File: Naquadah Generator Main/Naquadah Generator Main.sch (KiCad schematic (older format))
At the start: 15 parts, among them SW1 RESET, U1 ATmega32U4-AU, Y1 16MHz

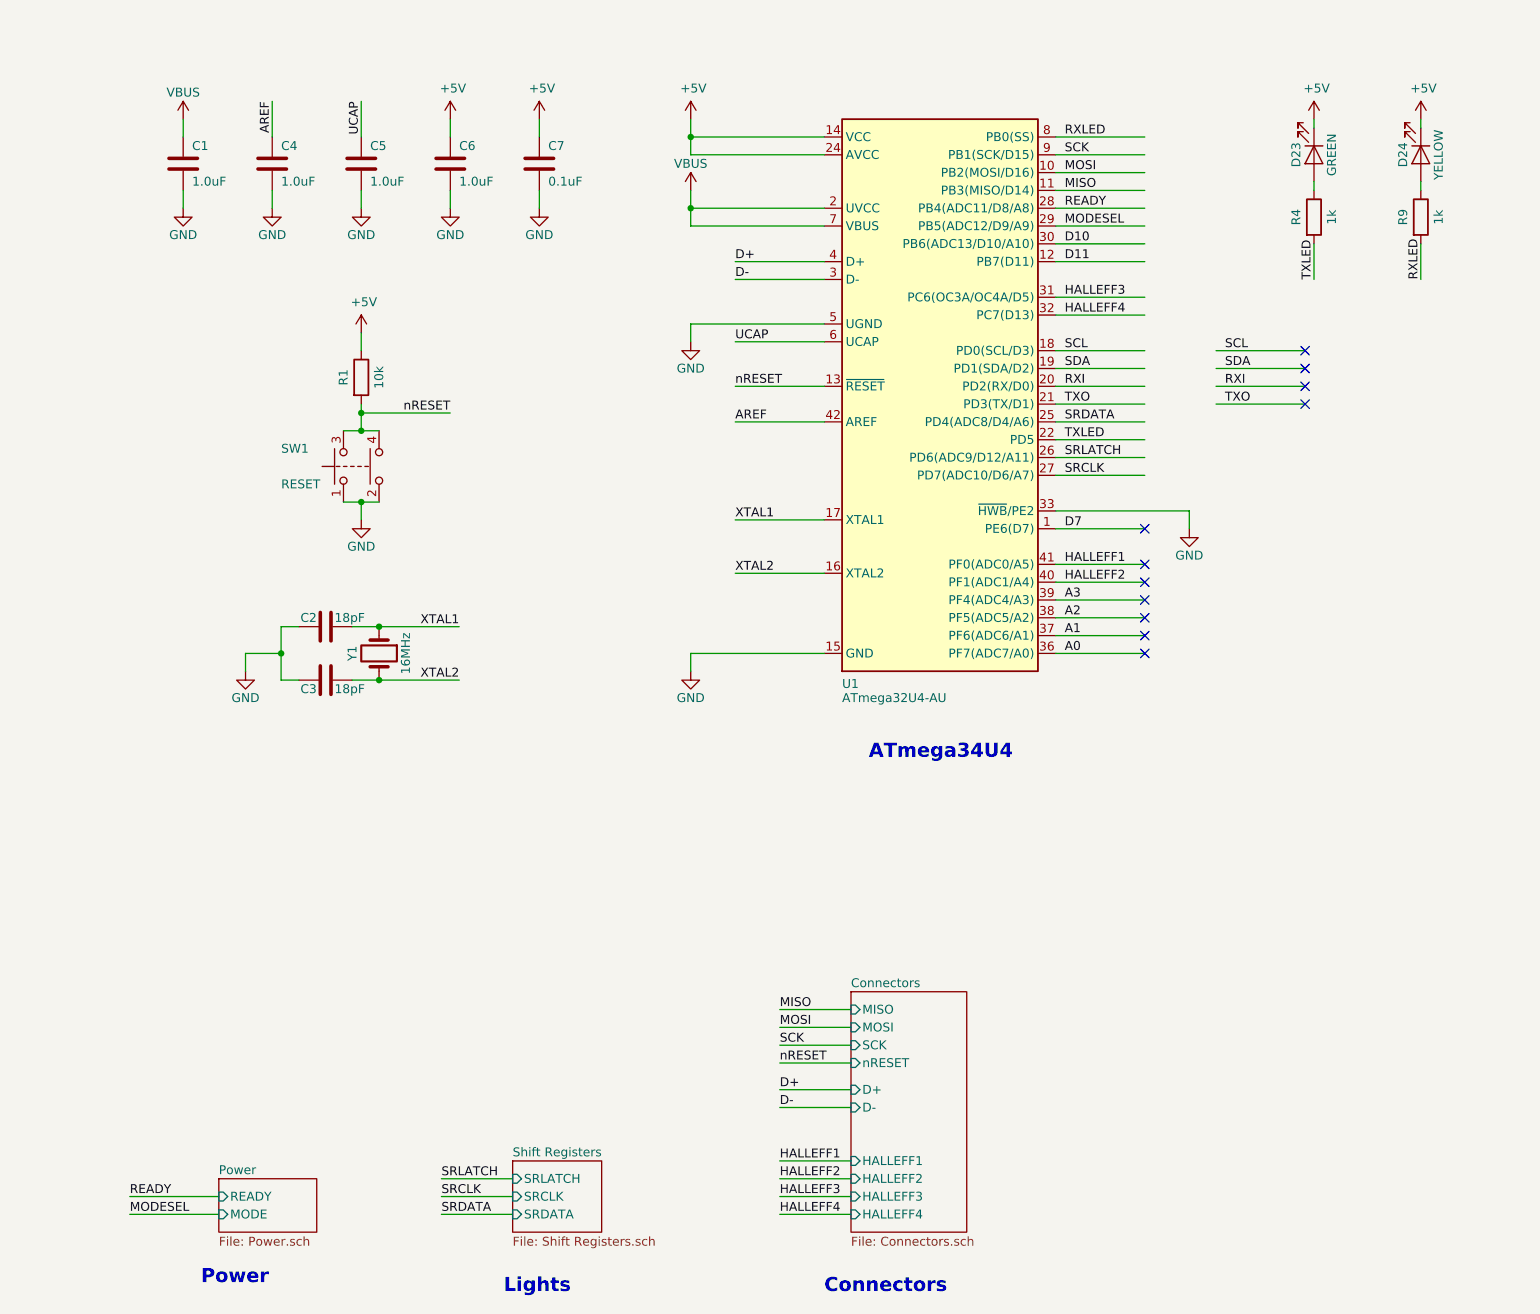
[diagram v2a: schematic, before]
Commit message: Updates
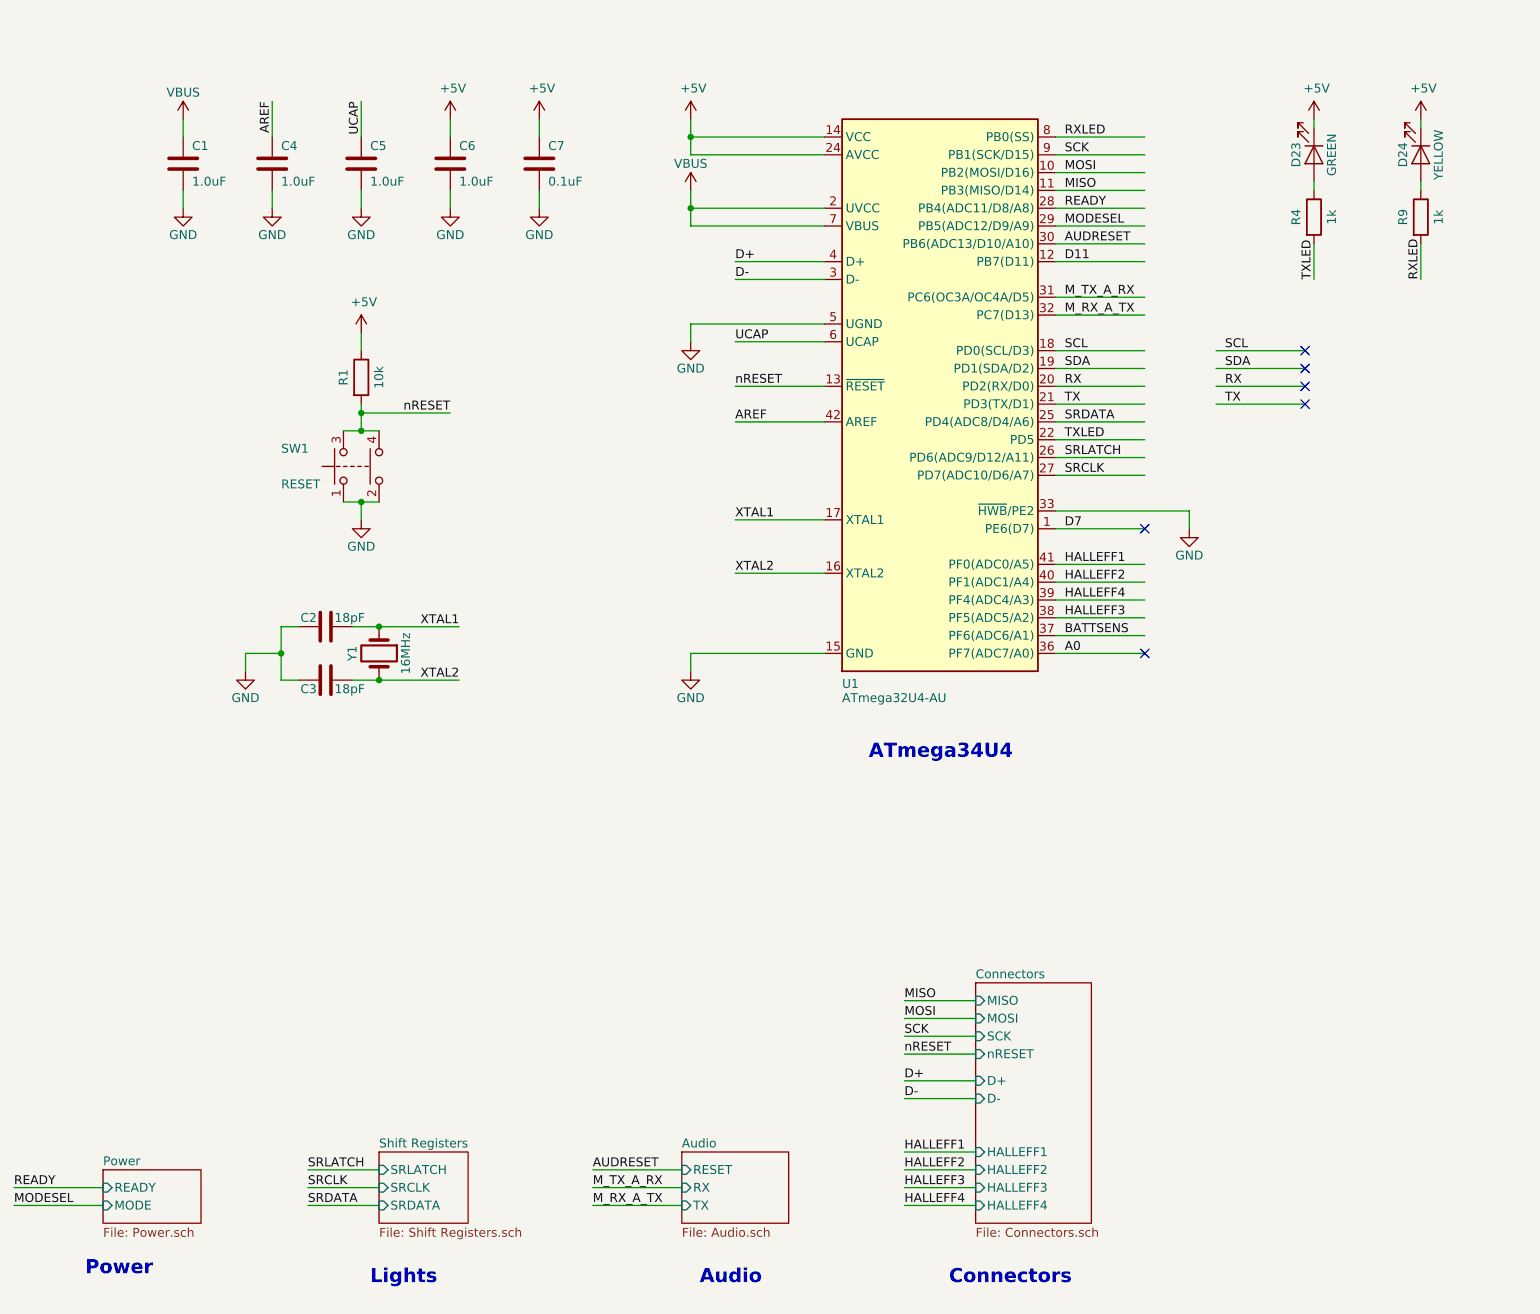
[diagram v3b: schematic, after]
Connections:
- net labels added: AUDRESET, BATTSENS, M_RX_A_TX, M_TX_A_RX, RX, TX
- net labels removed: A1, A2, A3, D10, RXI, TXO
- wire segments 100 -> 103
- no-connect marks 11 -> 6
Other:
- note added: "Audio"
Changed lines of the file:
@@
 $Descr A4 11693 8268
 encoding utf-8
-Sheet 1 11
+Sheet 1 12
 Title ""
 Date ""
@@
 	7050 3900 6550 3900
 Wire Wire Line
-	7050 3800 6550 3800
-Wire Wire Line
 	4750 2250 5250 2250
 Wire Wire Line
@@
 	4500 4000 4500 4100
 $Sheet
-S 3500 6850 500  400
+S 2750 6800 500  400
 U 5ED17BA0
 F0 "Shift Registers" 50
 F1 "Shift Registers.sch" 50
-F2 "SRLATCH" I L 3500 6950 50
-F3 "SRDATA" I L 3500 7150 50
-F4 "SRCLK" I L 3500 7050 50
+F2 "SRLATCH" I L 2750 6900 50
+F3 "SRDATA" I L 2750 7100 50
+F4 "SRCLK" I L 2750 7000 50
 $EndSheet
 Wire Wire Line
-	3500 6950 3100 6950
-Text Label 3100 6950 0    50   ~ 0
+	2750 6900 2350 6900
+Text Label 2350 6900 0    50   ~ 0
 SRLATCH
 Wire Wire Line
-	3500 7050 3100 7050
-Wire Wire Line
-	3500 7150 3100 7150
-Text Label 3100 7050 0    50   ~ 0
+	2750 7000 2350 7000
+Wire Wire Line
+	2750 7100 2350 7100
+Text Label 2350 7000 0    50   ~ 0
 SRCLK
 Wire Wire Line
@@
 Text Notes 5500 4600 0    79   ~ 16
 ATmega34U4
-Text Notes 3450 7600 0    79   ~ 16
+Text Notes 2700 7550 0    79   ~ 16
 Lights
 Wire Wire Line
@@
 Text Label 6600 1200 0    50   ~ 0
 SCK
-Text Notes 1750 7550 0    79   ~ 16
+Text Notes 1100 7500 0    79   ~ 16
 Power
-Text Label 3100 7150 0    50   ~ 0
+Text Label 2350 7100 0    50   ~ 0
 SRDATA
-Text Label 5000 6450 0    50   ~ 0
+Text Label 5700 6400 0    50   ~ 0
 D+
 Wire Wire Line
-	5000 6450 5400 6450
-Text Label 5000 6550 0    50   ~ 0
+	5700 6400 6100 6400
+Text Label 5700 6500 0    50   ~ 0
 D-
 Wire Wire Line
-	5000 6550 5400 6550
-Text Notes 5250 7600 0    79   ~ 16
+	5700 6500 6100 6500
+Text Notes 5950 7550 0    79   ~ 16
 Connectors
-Text Label 5000 6000 0    50   ~ 0
+Text Label 5700 5950 0    50   ~ 0
 MISO
 Wire Wire Line
-	5000 6000 5400 6000
+	5700 5950 6100 5950
 $Sheet
-S 5400 5900 650  1350
+S 6100 5850 650  1350
 U 5EDBBDC8
 F0 "Connectors" 50
 F1 "Connectors.sch" 50
-F2 "MOSI" I L 5400 6100 50
-F3 "MISO" I L 5400 6000 50
-F4 "SCK" I L 5400 6200 50
-F5 "nRESET" I L 5400 6300 50
-F6 "HALLEFF2" I L 5400 6950 50
-F7 "HALLEFF1" I L 5400 6850 50
-F8 "HALLEFF3" I L 5400 7050 50
-F9 "HALLEFF4" I L 5400 7150 50
-F10 "D+" I L 5400 6450 50
-F11 "D-" I L 5400 6550 50
+F2 "MOSI" I L 6100 6050 50
+F3 "MISO" I L 6100 5950 50
+F4 "SCK" I L 6100 6150 50
+F5 "nRESET" I L 6100 6250 50
+F6 "HALLEFF2" I L 6100 6900 50
+F7 "HALLEFF1" I L 6100 6800 50
+F8 "HALLEFF3" I L 6100 7000 50
+F9 "HALLEFF4" I L 6100 7100 50
+F10 "D+" I L 6100 6400 50
+F11 "D-" I L 6100 6500 50
 $EndSheet
-Text Label 5000 6200 0    50   ~ 0
+Text Label 5700 6150 0    50   ~ 0
 SCK
 Wire Wire Line
-	5000 6200 5400 6200
-Text Label 5000 6100 0    50   ~ 0
+	5700 6150 6100 6150
+Text Label 5700 6050 0    50   ~ 0
 MOSI
 Wire Wire Line
-	5000 6100 5400 6100
-Text Label 5000 6300 0    50   ~ 0
+	5700 6050 6100 6050
+Text Label 5700 6250 0    50   ~ 0
 nRESET
 Wire Wire Line
-	5000 6300 5400 6300
-Text Label 5000 7150 0    50   ~ 0
+	5700 6250 6100 6250
+Text Label 5700 7100 0    50   ~ 0
 HALLEFF4
-Text Label 5000 7050 0    50   ~ 0
+Text Label 5700 7000 0    50   ~ 0
 HALLEFF3
 Wire Wire Line
-	5400 7050 5000 7050
-Wire Wire Line
-	5400 7150 5000 7150
-Text Label 5000 6950 0    50   ~ 0
+	6100 7000 5700 7000
+Wire Wire Line
+	6100 7100 5700 7100
+Text Label 5700 6900 0    50   ~ 0
 HALLEFF2
-Text Label 5000 6850 0    50   ~ 0
+Text Label 5700 6800 0    50   ~ 0
 HALLEFF1
 Wire Wire Line
-	5400 6850 5000 6850
-Wire Wire Line
-	5400 6950 5000 6950
+	6100 6800 5700 6800
+Wire Wire Line
+	6100 6900 5700 6900
 Wire Wire Line
 	8000 1400 8000 1350
@@
 Wire Wire Line
 	7050 3700 6550 3700
-Text Label 6600 3700 0    50   ~ 0
-A3
 Text Label 6600 3300 0    50   ~ 0
 D7
@@
 	6550 1700 7050 1700
 Text Label 6600 1700 0    50   ~ 0
-D10
+AUDRESET
 Wire Wire Line
 	6550 2500 7050 2500
 Text Label 6600 2500 0    50   ~ 0
-RXI
+RX
 Wire Wire Line
 	6550 2600 7050 2600
 Text Label 6600 2600 0    50   ~ 0
-TXO
+TX
 $Sheet
-S 1850 6950 550  300
+S 1200 6900 550  300
 U 5EA6751D
 F0 "Power" 50
 F1 "Power.sch" 50
-F2 "READY" I L 1850 7050 50
-F3 "MODE" I L 1850 7150 50
+F2 "READY" I L 1200 7000 50
+F3 "MODE" I L 1200 7100 50
 $EndSheet
 Wire Wire Line
-	1350 7150 1850 7150
-Text Label 1350 7150 0    50   ~ 0
+	700  7100 1200 7100
+Text Label 700  7100 0    50   ~ 0
 MODESEL
 Wire Wire Line
-	1350 7050 1850 7050
-Text Label 1350 7050 0    50   ~ 0
+	700  7000 1200 7000
+Text Label 700  7000 0    50   ~ 0
 READY
 Text Label 3200 4150 2    50   ~ 0
@@
 HALLEFF2
 Text Label 6600 2100 0    50   ~ 0
-HALLEFF4
+M_RX_A_TX
 Wire Wire Line
 	6550 2900 7050 2900
@@
 SRDATA
 Text Label 6600 2000 0    50   ~ 0
-HALLEFF3
+M_TX_A_RX
 Text Label 6600 3500 0    50   ~ 0
 HALLEFF1
 Wire Wire Line
 	7050 3600 6550 3600
-Wire Wire Line
-	7050 3500 6550 3500
 NoConn ~ 7050 3300
-NoConn ~ 7050 3500
-NoConn ~ 7050 3600
-NoConn ~ 7050 3700
-NoConn ~ 7050 3800
-NoConn ~ 7050 3900
 NoConn ~ 7050 4000
 Wire Wire Line
@@
 Text Label 6600 2300 0    50   ~ 0
 SCL
-Text Label 6600 3800 0    50   ~ 0
-A2
 Text Label 6600 3900 0    50   ~ 0
-A1
+BATTSENS
 Text Label 6600 4000 0    50   ~ 0
 A0
@@
 	7450 2500 7950 2500
 Text Label 7500 2500 0    50   ~ 0
-RXI
+RX
 Wire Wire Line
 	7450 2600 7950 2600
 Text Label 7500 2600 0    50   ~ 0
-TXO
+TX
 Text Label 7500 2300 0    50   ~ 0
 SCL
@@
 NoConn ~ 7950 2500
 NoConn ~ 7950 2600
+Text Label 6600 3700 0    50   ~ 0
+HALLEFF4
+Text Label 6600 3800 0    50   ~ 0
+HALLEFF3
+Wire Wire Line
+	7050 3500 6550 3500
+Wire Wire Line
+	7050 3800 6550 3800
+$Sheet
+S 4450 6800 600  400
+U 5F06C1CA
+F0 "Audio" 50
+F1 "Audio.sch" 50
+F2 "RESET" I L 4450 6900 50
+F3 "RX" I L 4450 7000 50
+F4 "TX" I L 4450 7100 50
+$EndSheet
+Text Notes 4550 7550 0    79   ~ 16
+Audio
+Wire Wire Line
+	3950 7000 4450 7000
+Text Label 3950 7100 0    50   ~ 0
+M_RX_A_TX
+Text Label 3950 7000 0    50   ~ 0
+M_TX_A_RX
+Wire Wire Line
+	3950 7100 4450 7100
+Wire Wire Line
+	3950 6900 4450 6900
+Text Label 3950 6900 0    50   ~ 0
+AUDRESET
 $EndSCHEMATC

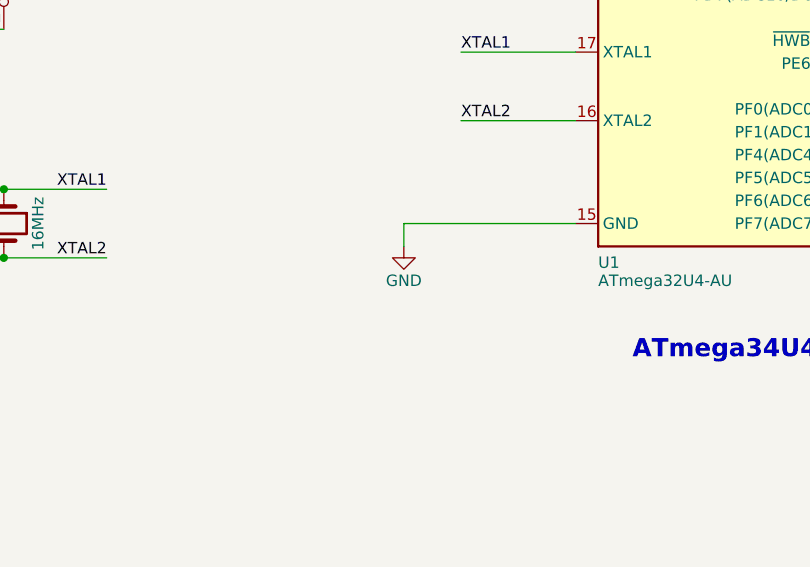
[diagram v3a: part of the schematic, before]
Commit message: Start of audio
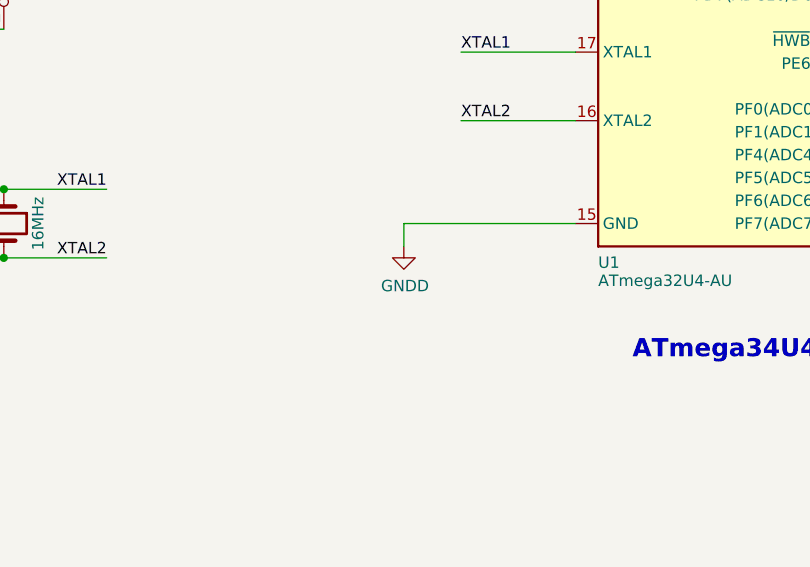
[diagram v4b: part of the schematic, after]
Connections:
- net labels added: GNDD
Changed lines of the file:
@@
 Wire Wire Line
 	6550 3000 7050 3000
-$Comp
-L Frequently_Used_LE:GND #PWR017
-U 1 1 5EA1BAA4
-P 4500 4100
-F 0 "#PWR017" H 4500 3850 50  0001 C CNN
-F 1 "GND" H 4500 3950 50  0000 C CNN
-F 2 "" H 4500 4100 50  0001 C CNN
-F 3 "" H 4500 4100 50  0001 C CNN
-	1    4500 4100
-	1    0    0    -1
-$EndComp
 Wire Wire Line
 	4500 4000 4500 4100
@@
 Text Label 3950 6900 0    50   ~ 0
 AUDRESET
+$Comp
+L Frequently_Used_LE:GNDD #PWR?
+U 1 1 5F267B9F
+P 4500 4100
+F 0 "#PWR?" H 4500 3850 50  0001 C CNN
+F 1 "GNDD" H 4505 3927 50  0000 C CNN
+F 2 "" H 4500 4100 50  0001 C CNN
+F 3 "" H 4500 4100 50  0001 C CNN
+	1    4500 4100
+	1    0    0    -1
+$EndComp
 $EndSCHEMATC
